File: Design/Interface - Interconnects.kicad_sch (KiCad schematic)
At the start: 0 parts

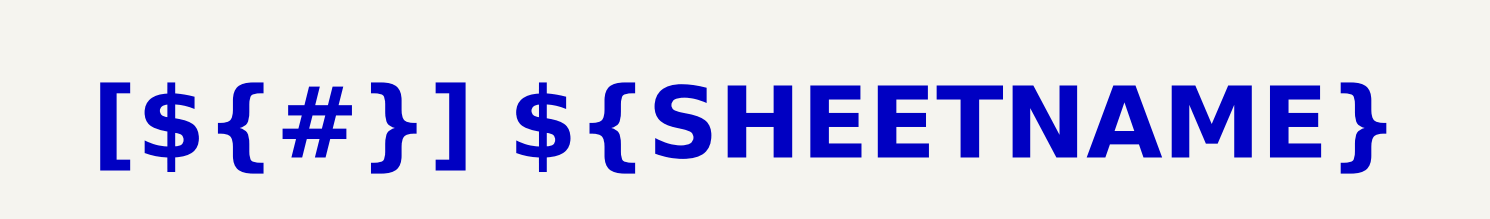
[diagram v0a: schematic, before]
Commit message: new frame work for the design
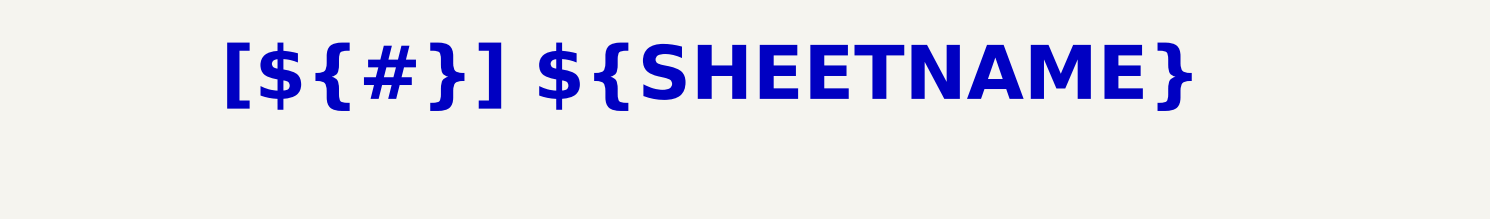
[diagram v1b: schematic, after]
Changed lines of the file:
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@@
 	(text "[${#}] ${SHEETNAME}"
 		(exclude_from_sim no)
-		(at 140.716 22.86 0)
+		(at 136.906 17.272 0)
 		(effects
 			(font
 				(face "Times New Roman")
-				(size 8 8)
+				(size 6 6)
 				(thickness 1.6)
 				(bold yes)
